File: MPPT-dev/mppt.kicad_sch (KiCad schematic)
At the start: 26 parts, among them Q1 PMOS, U1 LTC4412xS6, U2 LT8611EUDD-PBF, U3 AD5245BRJZ10-R2

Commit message: 1 mppt layout
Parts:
- Q1: footprint footprints:TO252_DMP6180SK3_DIO -> Package_SO:PowerPAK_SO-8_Single
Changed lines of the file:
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@@
 			)
 		)
-		(property "Footprint" "footprints:TO252_DMP6180SK3_DIO"
+		(property "Footprint" "Package_SO:PowerPAK_SO-8_Single"
 			(at 110.49 113.03 0)
 			(effects

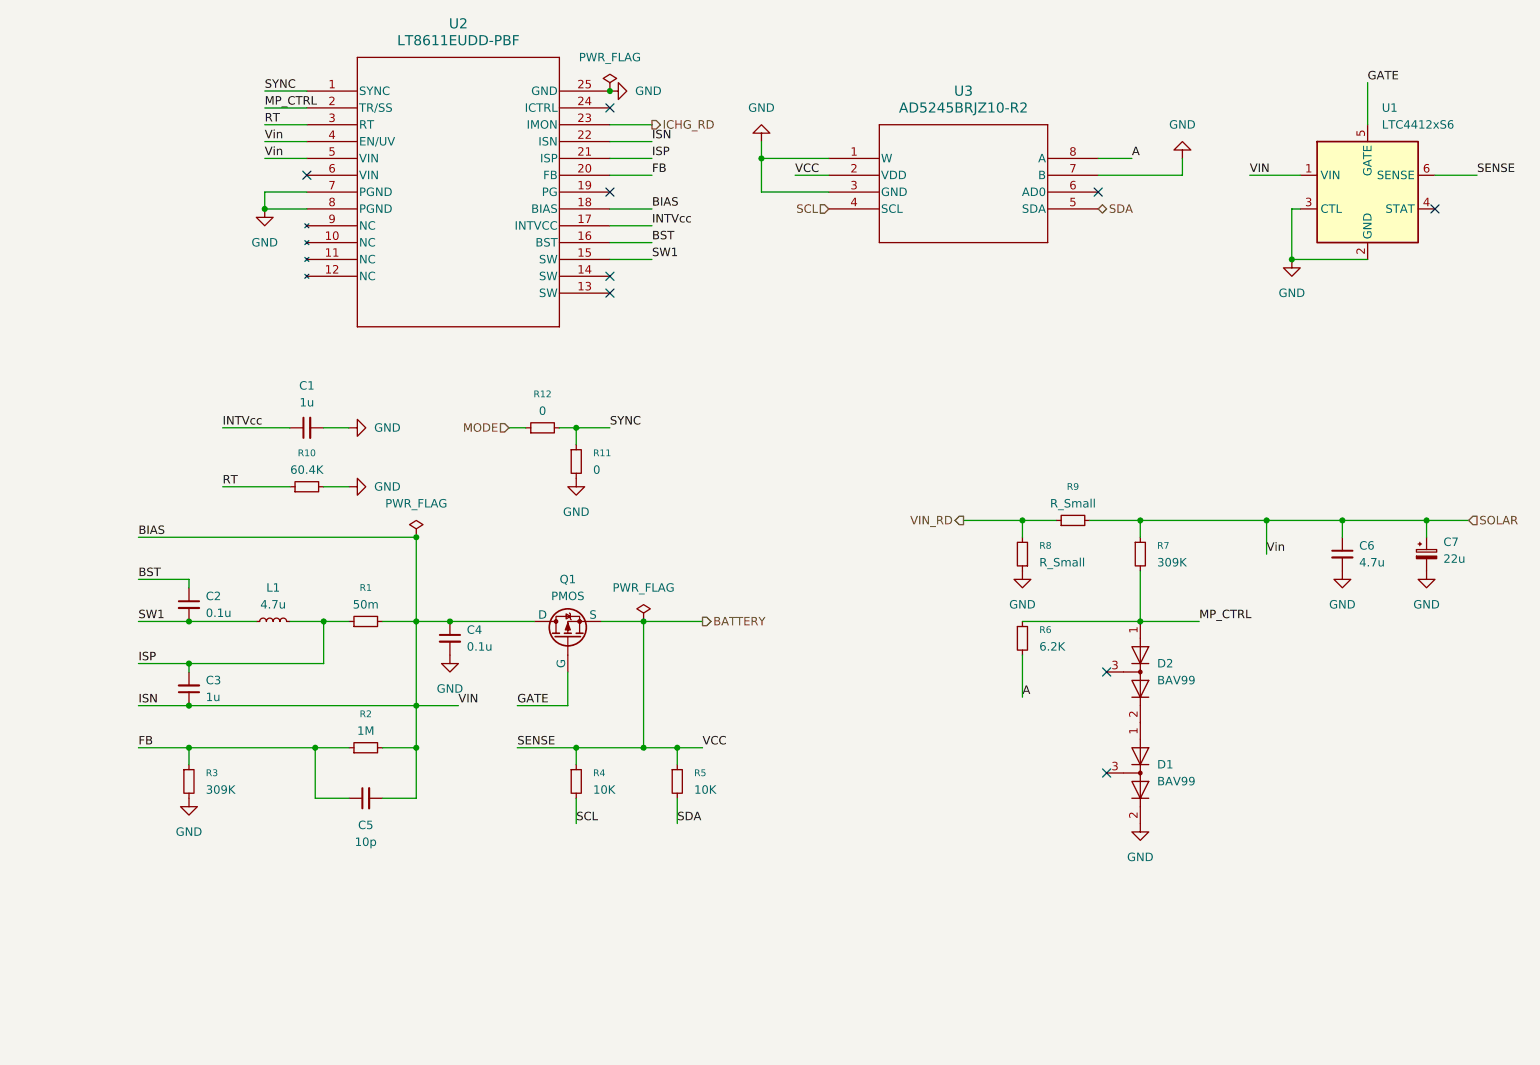
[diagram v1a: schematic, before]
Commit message: Board review
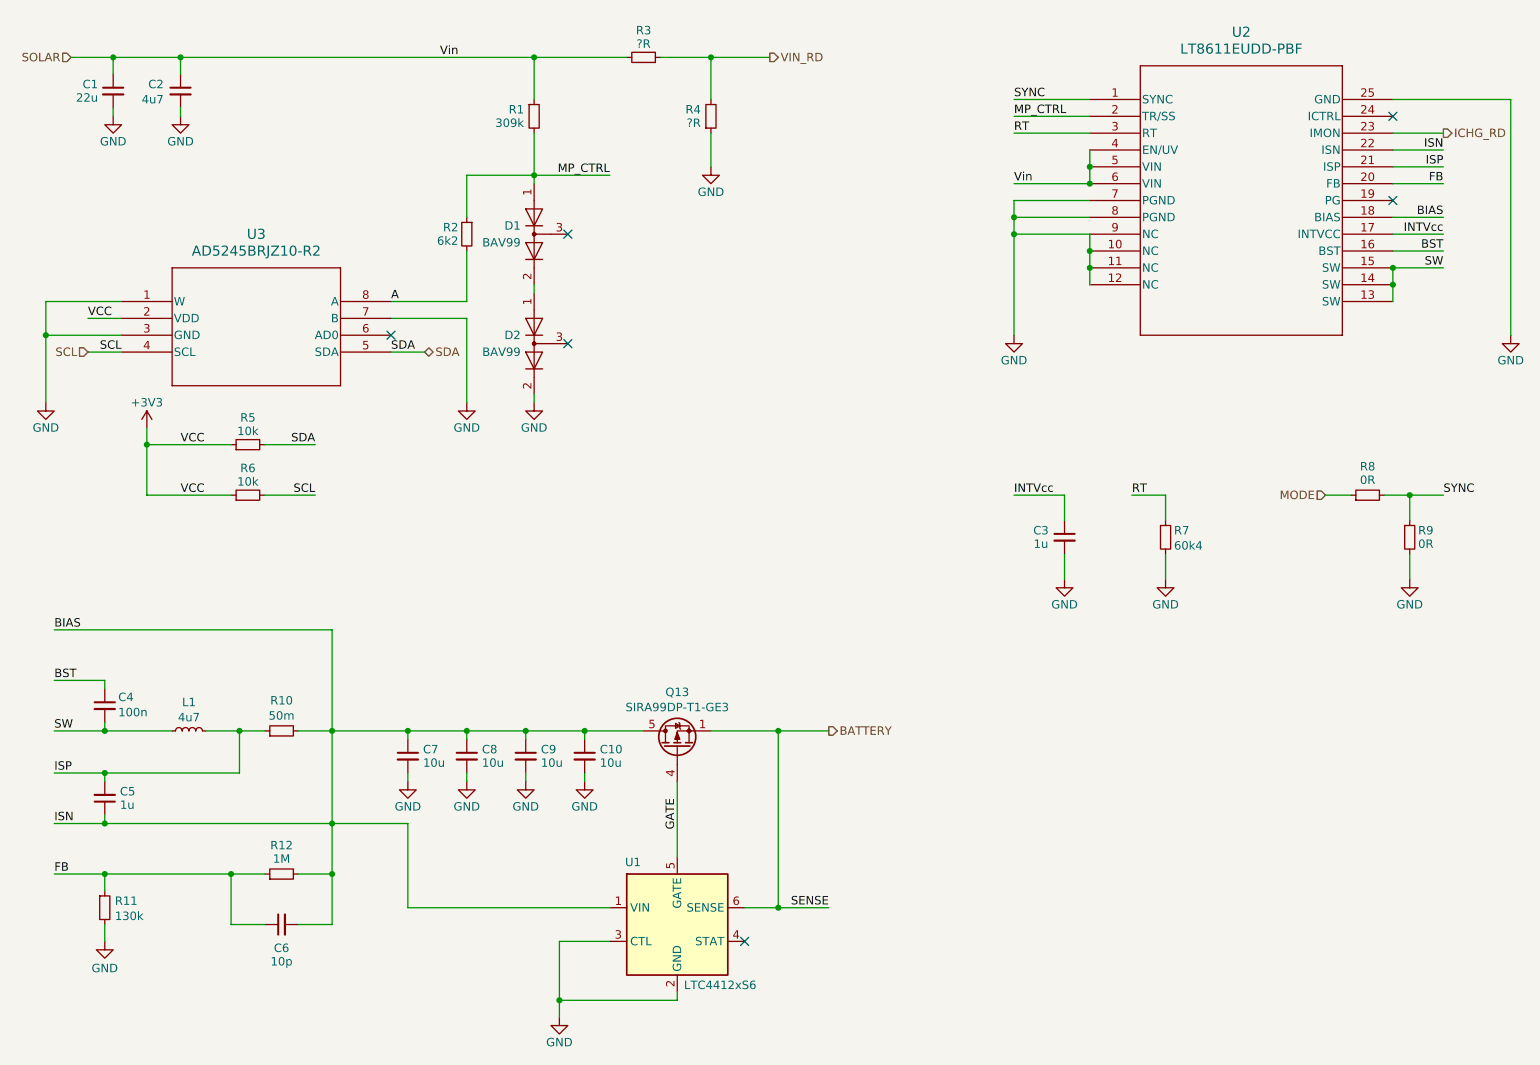
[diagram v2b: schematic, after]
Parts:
- removed Q1: PMOS, Package_SO:PowerPAK_SO-8_Single, symbol Simulation_SPICE:PMOS
- removed R4: 10K, Resistor_SMD:R_0805_2012Metric, symbol Device:R_Small
- added C10, C8, C9: 10u, Capacitor_SMD:C_0603_1608Metric, symbol Device:C_Small
- added Q13: SIRA99DP-T1-GE3, Package_SO:PowerPAK_SO-8_Single, symbol Transistor_FET:Si7141DP
- added R6: 10k, Resistor_SMD:R_0603_1608Metric, symbol Device:R_Small
- C1: renamed from C7; footprint Capacitor_SMD:C_0805_2012Metric -> Capacitor_SMD:C_0603_1608Metric; symbol Device:C_Polarized_Small -> Device:C_Small
- C2: renamed from C6; value 4.7u -> 4u7; footprint Capacitor_SMD:C_0805_2012Metric -> Capacitor_SMD:C_0603_1608Metric
- C3: renamed from C1; footprint Capacitor_SMD:C_0805_2012Metric -> Capacitor_SMD:C_0603_1608Metric
- C4: renamed from C2; value 0.1u -> 100n; footprint Capacitor_SMD:C_0805_2012Metric -> Capacitor_SMD:C_0603_1608Metric
- C5: renamed from C3; footprint Capacitor_SMD:C_0805_2012Metric -> Capacitor_SMD:C_0603_1608Metric
- C6: renamed from C5; footprint Capacitor_SMD:C_0805_2012Metric -> Capacitor_SMD:C_0603_1608Metric
- C7: renamed from C4; value 0.1u -> 10u; footprint Capacitor_SMD:C_0805_2012Metric -> Capacitor_SMD:C_0603_1608Metric
- L1: value 4.7u -> 4u7; footprint Inductor_SMD:L_0805_2012Metric -> footprints:IND_03-4R7-R_EAT
- R1: renamed from R7; value 309K -> 309k; footprint Resistor_SMD:R_0805_2012Metric -> Resistor_SMD:R_0603_1608Metric
- R10: renamed from R1; footprint Resistor_SMD:R_0805_2012Metric -> Resistor_SMD:R_0603_1608Metric
- R11: renamed from R3; value 309K -> 130k; footprint Resistor_SMD:R_0805_2012Metric -> Resistor_SMD:R_0603_1608Metric
- R12: renamed from R2; footprint Resistor_SMD:R_0805_2012Metric -> Resistor_SMD:R_0603_1608Metric
- R2: renamed from R6; value 6.2K -> 6k2; footprint Resistor_SMD:R_0805_2012Metric -> Resistor_SMD:R_0603_1608Metric
- R3: renamed from R9; value R_Small -> ?R; footprint Resistor_SMD:R_0805_2012Metric -> Resistor_SMD:R_0603_1608Metric
- R4: renamed from R8; value R_Small -> ?R; footprint Resistor_SMD:R_0805_2012Metric -> Resistor_SMD:R_0603_1608Metric
- R5: value 10K -> 10k; footprint Resistor_SMD:R_0805_2012Metric -> Resistor_SMD:R_0603_1608Metric
- R7: renamed from R10; value 60.4K -> 60k4; footprint Resistor_SMD:R_0805_2012Metric -> Resistor_SMD:R_0603_1608Metric
- R8: renamed from R12; value 0 -> 0R; footprint Resistor_SMD:R_0805_2012Metric -> Resistor_SMD:R_0603_1608Metric
- R9: renamed from R11; value 0 -> 0R; footprint Resistor_SMD:R_0805_2012Metric -> Resistor_SMD:R_0603_1608Metric
- U3: footprint RJ_8_ADI -> footprints:RJ_8_ADI
- renumbered D2 to D1, D1 to D2
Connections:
- net SW1 is gone; now on net SW: C4.2, L1.1, U2.15 (SW)
- net BATTERY: now also Q13.1 (S), Q13.2 (S), Q13.3 (S); no longer R5.1, U3.2 (VDD)
- net BIAS: now also C10.1, C8.1, C9.1, Q13.5 (D)
- net GATE: now also Q13.4 (G)
- net GND: now also U2.10 (NC), U2.11 (NC), U2.12 (NC), U2.9 (NC), C10.2, C8.2, C9.2
- net SCL: now also R6.2
- net SOLAR: now also U2.6 (VIN)
- net SW: now reaches U2.13 (SW)
- net SW: now also U2.14 (SW)
- new net +3V3: R5.1, R6.1, U3.2 (VDD)
- no-connect marks 9 -> 6
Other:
- moved on the sheet: C2, C3, C4, C5, C6, C7, D1, D2, L1, R1, R10, R11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
